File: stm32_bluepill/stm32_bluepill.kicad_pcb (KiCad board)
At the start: 2 copper layers, 8.7 x 30 mm, 33 parts, among them J1 USB_B_Micro, J2 Conn_01x04_Pin, J4 Conn_01x04_Pin, J5 Conn_01x04_Pin, J6 Conn_01x08_Pin, SW1 SW_SPDT, U1 STM32F103C8T6, U2 AMS1117-3.3, Y1 16MHz

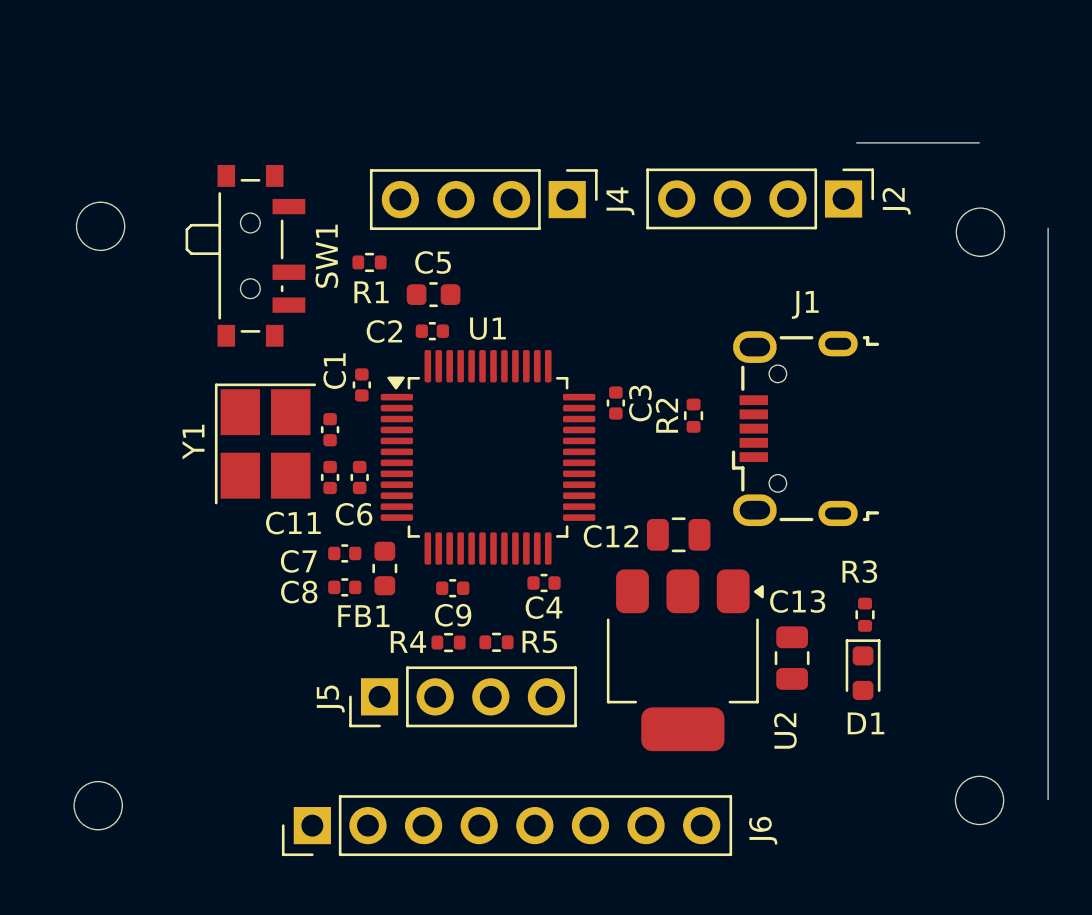
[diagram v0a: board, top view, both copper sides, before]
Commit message: Add files via upload
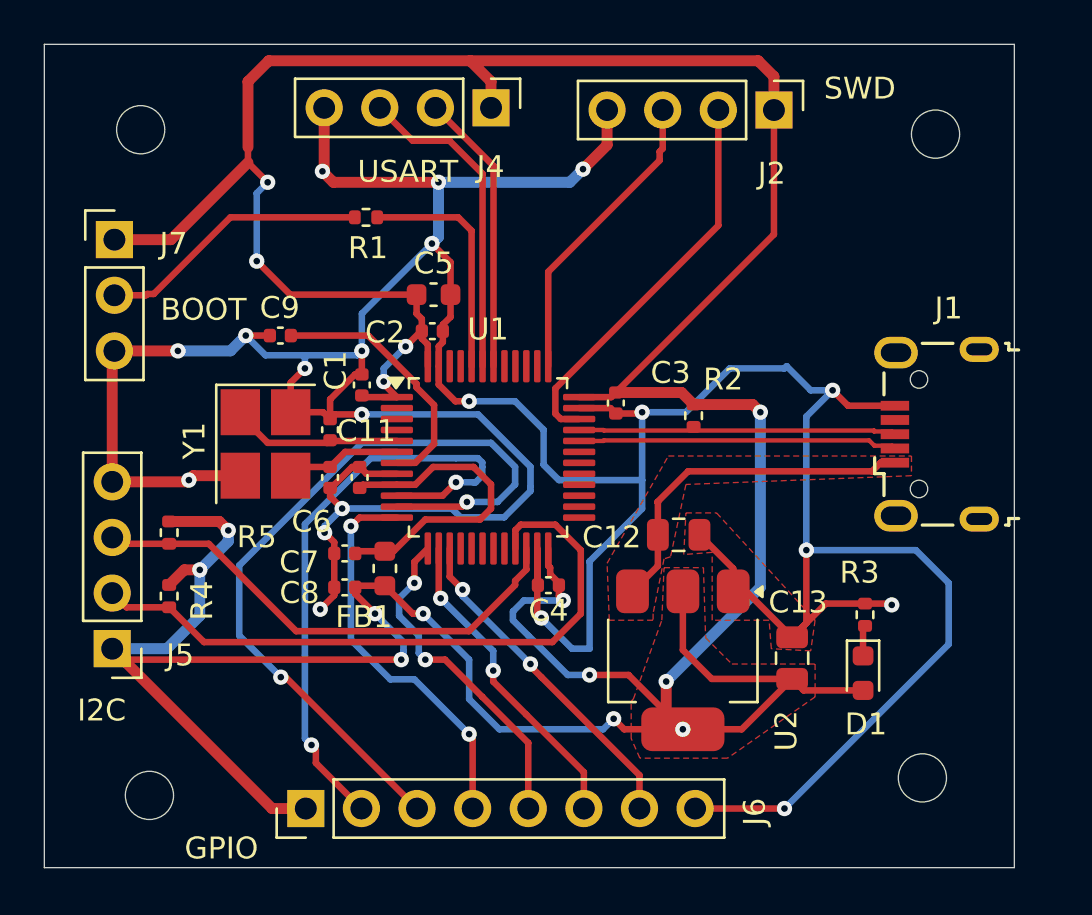
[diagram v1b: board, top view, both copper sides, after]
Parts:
- removed SW1: SW_SPDT, Button_Switch_SMD:SW_SPDT_PCM12
- added J7: Conn_01x03_Pin, Connector_PinHeader_2.54mm:PinHeader_1x03_P2.54mm_Vertical, F.Cu at (99.6, 40.7)
- moved R5 15.8 mm to (102.1, 54.1), turned to 90 degrees
- moved C9 14.0 mm to (107.2, 45.1), turned to 180 degrees
- moved R4 12.9 mm to (102.1, 57.0), turned to 90 degrees
- moved J5 12.4 mm to (99.5, 59.4), turned to 180 degrees
- moved J1 6.45 mm to (137.1, 49.6)
- moved J4 5.45 mm to (116.8, 34.7)
- moved J2 5.16 mm to (129.7, 34.8)
- moved H1 4.93 mm to (137.1, 35.9)
- moved H3 4.77 mm to (100.8, 35.7)
- moved H2 2.81 mm to (136.5, 65.3)
- moved H4 2.39 mm to (101.2, 66.1)
- moved R1 2.07 mm to (111.1, 39.7)
- moved J6 0.84 mm to (108.3, 66.7)
- moved C4 0.22 mm to (119.4, 56.5)
- turned C11 to -90 degrees
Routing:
- net +3.3V: track 0.00 -> 198.7 mm, vias 0 -> 15
- net GND: track 0.00 -> 196.0 mm, vias 0 -> 20
- net /GPIO_1: track 0.00 -> 36.6 mm, vias 0 -> 2
- net /I2C2_SCL: track 0.00 -> 30.2 mm
- net /GPIO_0: track 0.00 -> 28.4 mm, vias 0 -> 2
- net /I2C2_SDA: track 0.00 -> 22.9 mm
- net /SWDIO: track 0.00 -> 18.1 mm
- net /GPIO_2: track 0.00 -> 18.1 mm, vias 0 -> 2
- net VBUS: track 0.00 -> 16.2 mm
- net /GPIO_5: track 0.00 -> 15.5 mm, vias 0 -> 2
- net /GPIO_3: track 0.00 -> 15.4 mm, vias 0 -> 2
- net +3.3VA: track 0.00 -> 14.9 mm
- net /USART1_RX: track 0.00 -> 14.7 mm
- net /GPIO_4: track 0.00 -> 14.6 mm, vias 0 -> 2
- net /USB_D-: track 0.00 -> 14.6 mm
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- added copper zone on F.Cu, net +3.3V
- added copper zone on F.Cu, net GND
- added copper zone on F.Cu, net VBUS
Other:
- board size 8.7 x 30 mm -> 44.3 x 37.6 mm
- board text added: "BOOT"
- board text added: "GPIO"
- board text added: "I2C"
- board text added: "SWD"
- board text added: "USART"
